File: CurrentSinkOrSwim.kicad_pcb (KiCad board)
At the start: 2 copper layers, 41.7 x 47.8 mm, 23 parts, among them P1 CONN_01X01, P101 CONN_01X02, P102 CONN_01X03, P103 CONN_01X02, Q401 BUK9575, U201 LMV358, U301 LM2931D-R

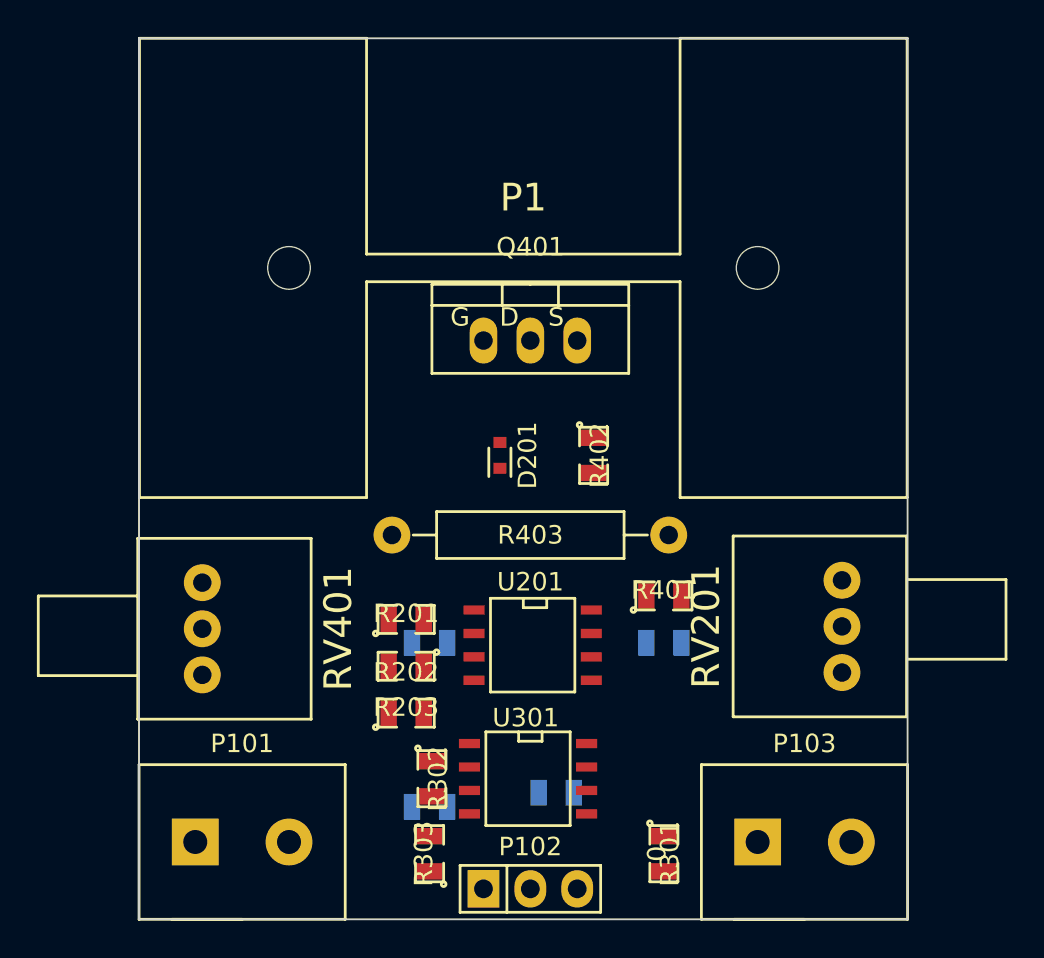
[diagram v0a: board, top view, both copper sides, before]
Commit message: CSOS Layout session 1
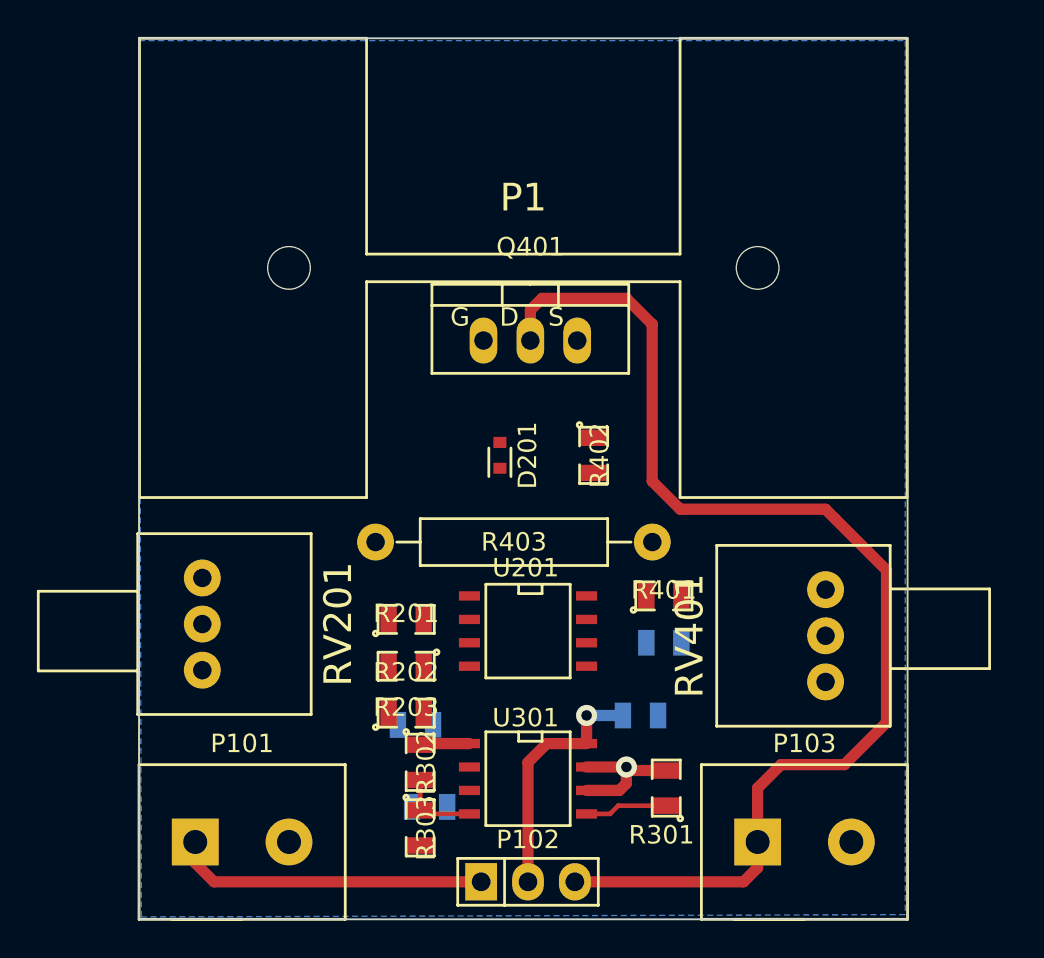
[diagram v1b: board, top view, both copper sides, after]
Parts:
- moved RV201 34.7 mm to (109.6, 67.6), turned to 270 degrees
- moved RV401 33.8 mm to (143.4, 68.2), turned to 90 degrees
- moved C301 12.1 mm to (133.3, 72.5)
- moved C302 8.46 mm to (121.2, 73.0), turned to 180 degrees
- moved R301 3.56 mm to (134.7, 76.5), turned to 90 degrees
- moved R303 1.49 mm to (121.4, 78.6), turned to 270 degrees
- moved R302 1.09 mm to (121.4, 75.1)
- moved R403 0.97 mm to (126.5, 63.1)
- moved U201 0.80 mm to (127.3, 67.9)
- moved P102 0.40 mm to (127.3, 81.5)
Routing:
- net /Current Control/Current_Sink+: track 0.00 -> 63.6 mm
- net Net-(P101-Pad1): track 0.00 -> 17.1 mm
- net /Power Regulation/Vin: track 0.00 -> 13.6 mm, vias 0 -> 1
- net GND: track 0.00 -> 7.60 mm, vias 0 -> 1
- net Net-(R301-Pad1): track 0.00 -> 4.50 mm
- net Net-(R302-Pad2): track 0.00 -> 4.40 mm
- net 2.7V: track 0.00 -> 2.69 mm
- added copper zone on B.Cu, net GND
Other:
- net class Power added: clearance 0.3048, trace_width 0.6096, via_dia 1.143, via_drill 0.762
